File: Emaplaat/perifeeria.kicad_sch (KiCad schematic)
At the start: 29 parts, among them J3 Conn_01x05_Socket, Q1 2N7002K

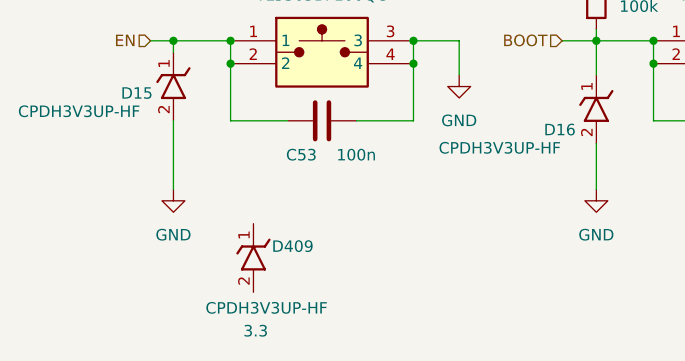
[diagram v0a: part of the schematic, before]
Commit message: v1.1 kuid veel pooleli
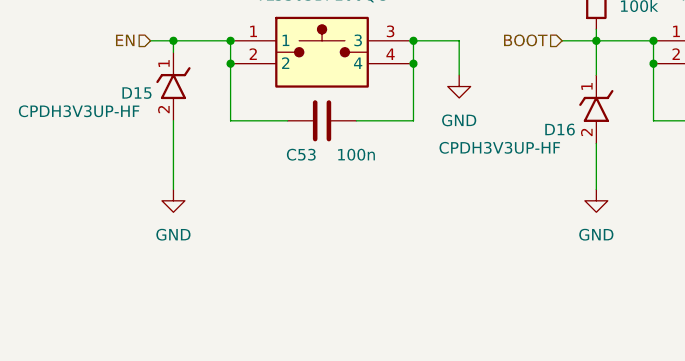
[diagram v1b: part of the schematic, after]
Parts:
- removed D409: CPDH3V3UP-HF, Diode_SMD:D_SOD-523, symbol CPDH3V3UP-HF:CPDH3V3UP-HF
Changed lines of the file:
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@@
-	)
-	(symbol
-		(lib_name "CPDH3V3UP-HF_2")
-		(lib_id "CPDH3V3UP-HF:CPDH3V3UP-HF")
-		(at 59.69 165.1 270)
-		(unit 1)
-		(exclude_from_sim no)
-		(in_bom yes)
-		(on_board yes)
-		(dnp no)
-		(property "Reference" "D409"
-			(at 61.722 172.72 90)
-			(effects
-				(font
-					(size 1.27 1.27)
-				)
-				(justify left)
-			)
-		)
-		(property "Value" "CPDH3V3UP-HF"
-			(at 54.356 179.578 90)
-			(effects
-				(font
-					(size 1.27 1.27)
-				)
-				(justify left)
-			)
-		)
-		(property "Footprint" "Diode_SMD:D_SOD-523"
-			(at -33.96 175.26 0)
-			(effects
-				(font
-					(size 1.27 1.27)
-				)
-				(justify left bottom)
-				(hide yes)
-			)
-		)
-		(property "Datasheet" "https://datasheet.datasheetarchive.com/originals/distributors/Datasheets-DGA26/1842371.pdf"
-			(at -133.96 175.26 0)
-			(effects
-				(font
-					(size 1.27 1.27)
-				)
-				(justify left bottom)
-				(hide yes)
-			)
-		)
-		(property "Description" "ESD Suppressors / TVS Diodes 5.5V, 15Kv"
-			(at 73.406 164.846 0)
-			(effects
-				(font
-					(size 1.27 1.27)
-				)
-				(hide yes)
-			)
-		)
-		(property "Height" "0.77"
-			(at -333.96 175.26 0)
-			(effects
-				(font
-					(size 1.27 1.27)
-				)
-				(justify left bottom)
-				(hide yes)
-			)
-		)
-		(property "Mouser Part Number" "750-CPDH3V3UP-HF"
-			(at -433.96 175.26 0)
-			(effects
-				(font
-					(size 1.27 1.27)
-				)
-				(justify left bottom)
-				(hide yes)
-			)
-		)
-		(property "Mouser Price/Stock" "https://www.mouser.co.uk/ProductDetail/Comchip-Technology/CPDH3V3UP-HF?qs=XEIV%2Fho1H6em2DT135enQw%3D%3D"
-			(at -533.96 175.26 0)
-			(effects
-				(font
-					(size 1.27 1.27)
-				)
-				(justify left bottom)
-				(hide yes)
-			)
-		)
-		(property "Manufacturer_Name" "Comchip Technology"
-			(at -633.96 175.26 0)
-			(effects
-				(font
-					(size 1.27 1.27)
-				)
-				(justify left bottom)
-				(hide yes)
-			)
-		)
-		(property "Manufacturer_Part_Number" "CPDH3V3UP-HF"
-			(at -733.96 175.26 0)
-			(effects
-				(font
-					(size 1.27 1.27)
-				)
-				(justify left bottom)
-				(hide yes)
-			)
-		)
-		(property "Voltage" "3.3"
-			(at 59.944 182.118 90)
-			(effects
-				(font
-					(size 1.27 1.27)
-				)
-			)
-		)
-		(pin "2"
-		)
-		(pin "1"
-		)
-		(instances
-			(project "Emaplaat"
-				(path "/489224c0-ace1-4530-aa61-a5d03adf1434/ac5852bd-1625-445e-9b6b-b65a0daab019"
-					(reference "D409")
-					(unit 1)
-				)
-			)
-		)
 	)
 	(symbol
